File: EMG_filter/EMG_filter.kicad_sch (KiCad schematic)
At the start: 16 parts, among them J1 Conn_01x03_Pin, J2 Conn_01x03_Pin, J3 Conn_01x04_Pin, U1 AD620, U2 MCP6022

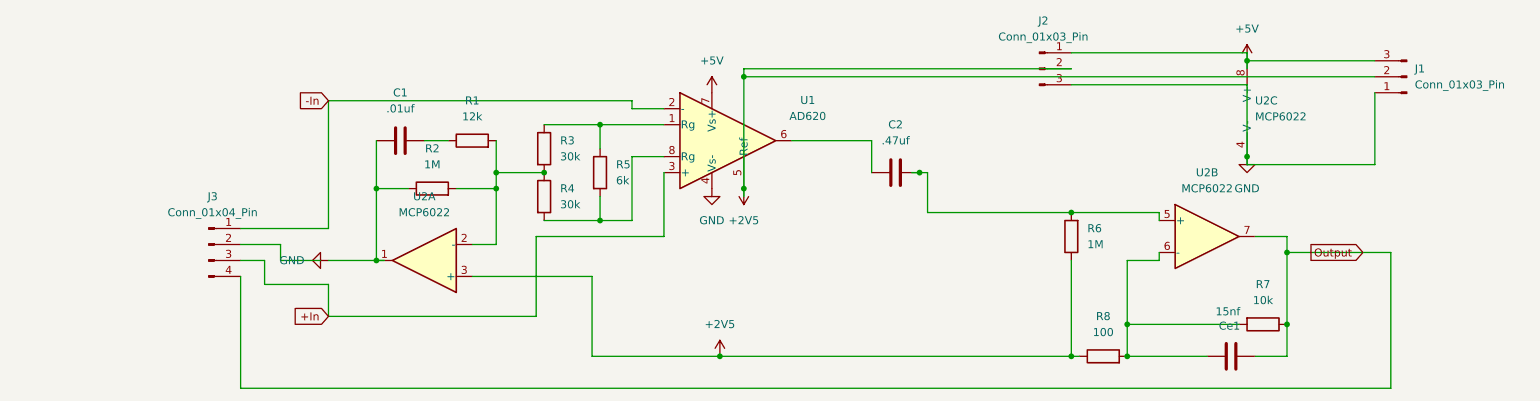
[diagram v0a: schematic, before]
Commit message: new filter
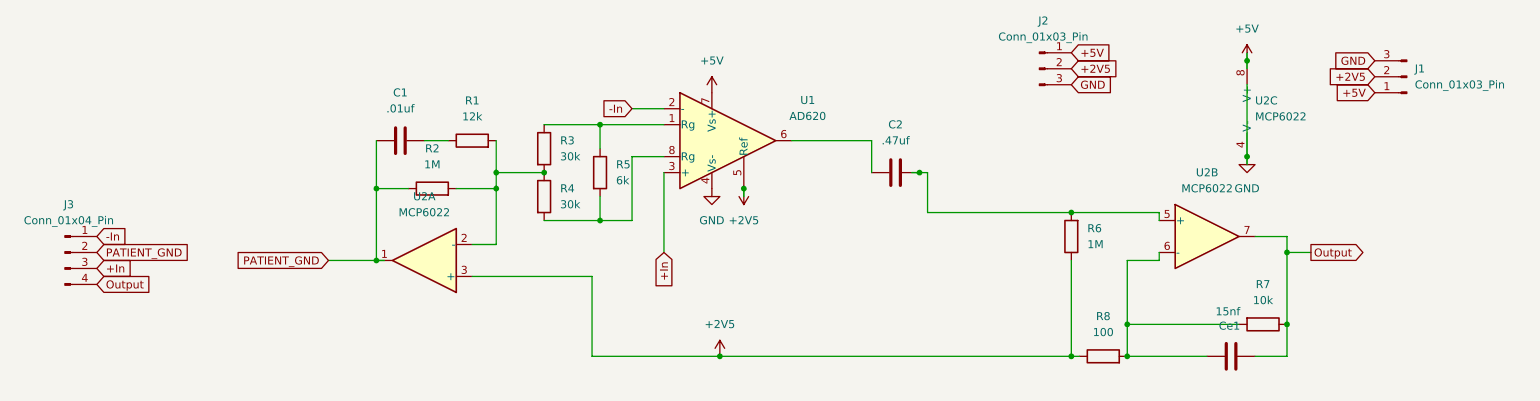
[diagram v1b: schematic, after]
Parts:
- U1, U2: footprint Package_SO:SOIC-8-1EP_3.9x4.9mm_P1.27mm_EP2.29x3mm -> Package_DIP:DIP-8_W7.62mm
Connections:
- net +5V: now also J1.1 (Pin_1); no longer J1.3 (Pin_3)
- net GND: now also J1.3 (Pin_3); no longer C1.1, J1.1 (Pin_1), R2.1, U2.1
- net PATIENT_GND: now reaches J3.2 (Pin_2)
- net PATIENT_GND: now also C1.1, R2.1, U2.1
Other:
- moved on the sheet: J3
